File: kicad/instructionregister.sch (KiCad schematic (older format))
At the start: 11 parts, among them U15 74LS173, U16 74LS173, U17 74LS245

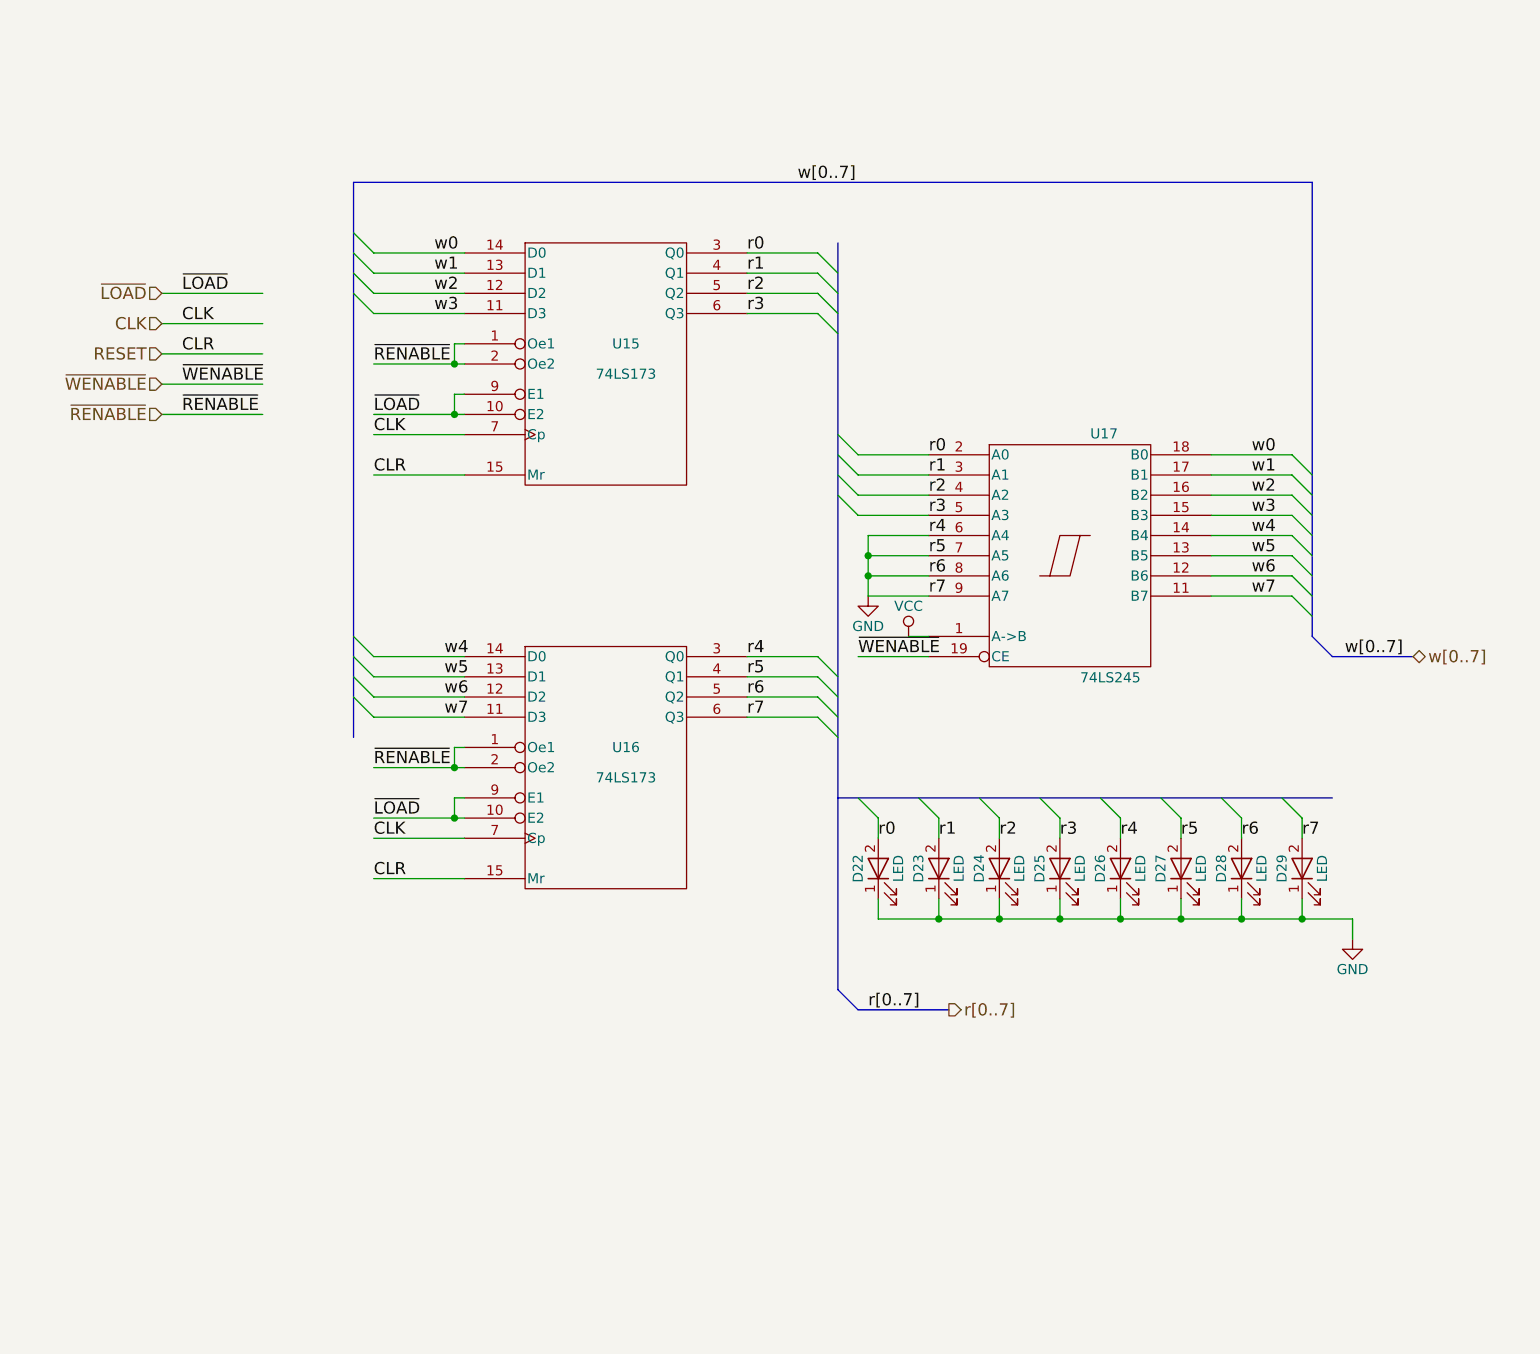
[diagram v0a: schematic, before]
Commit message: Update to current kicad libraries
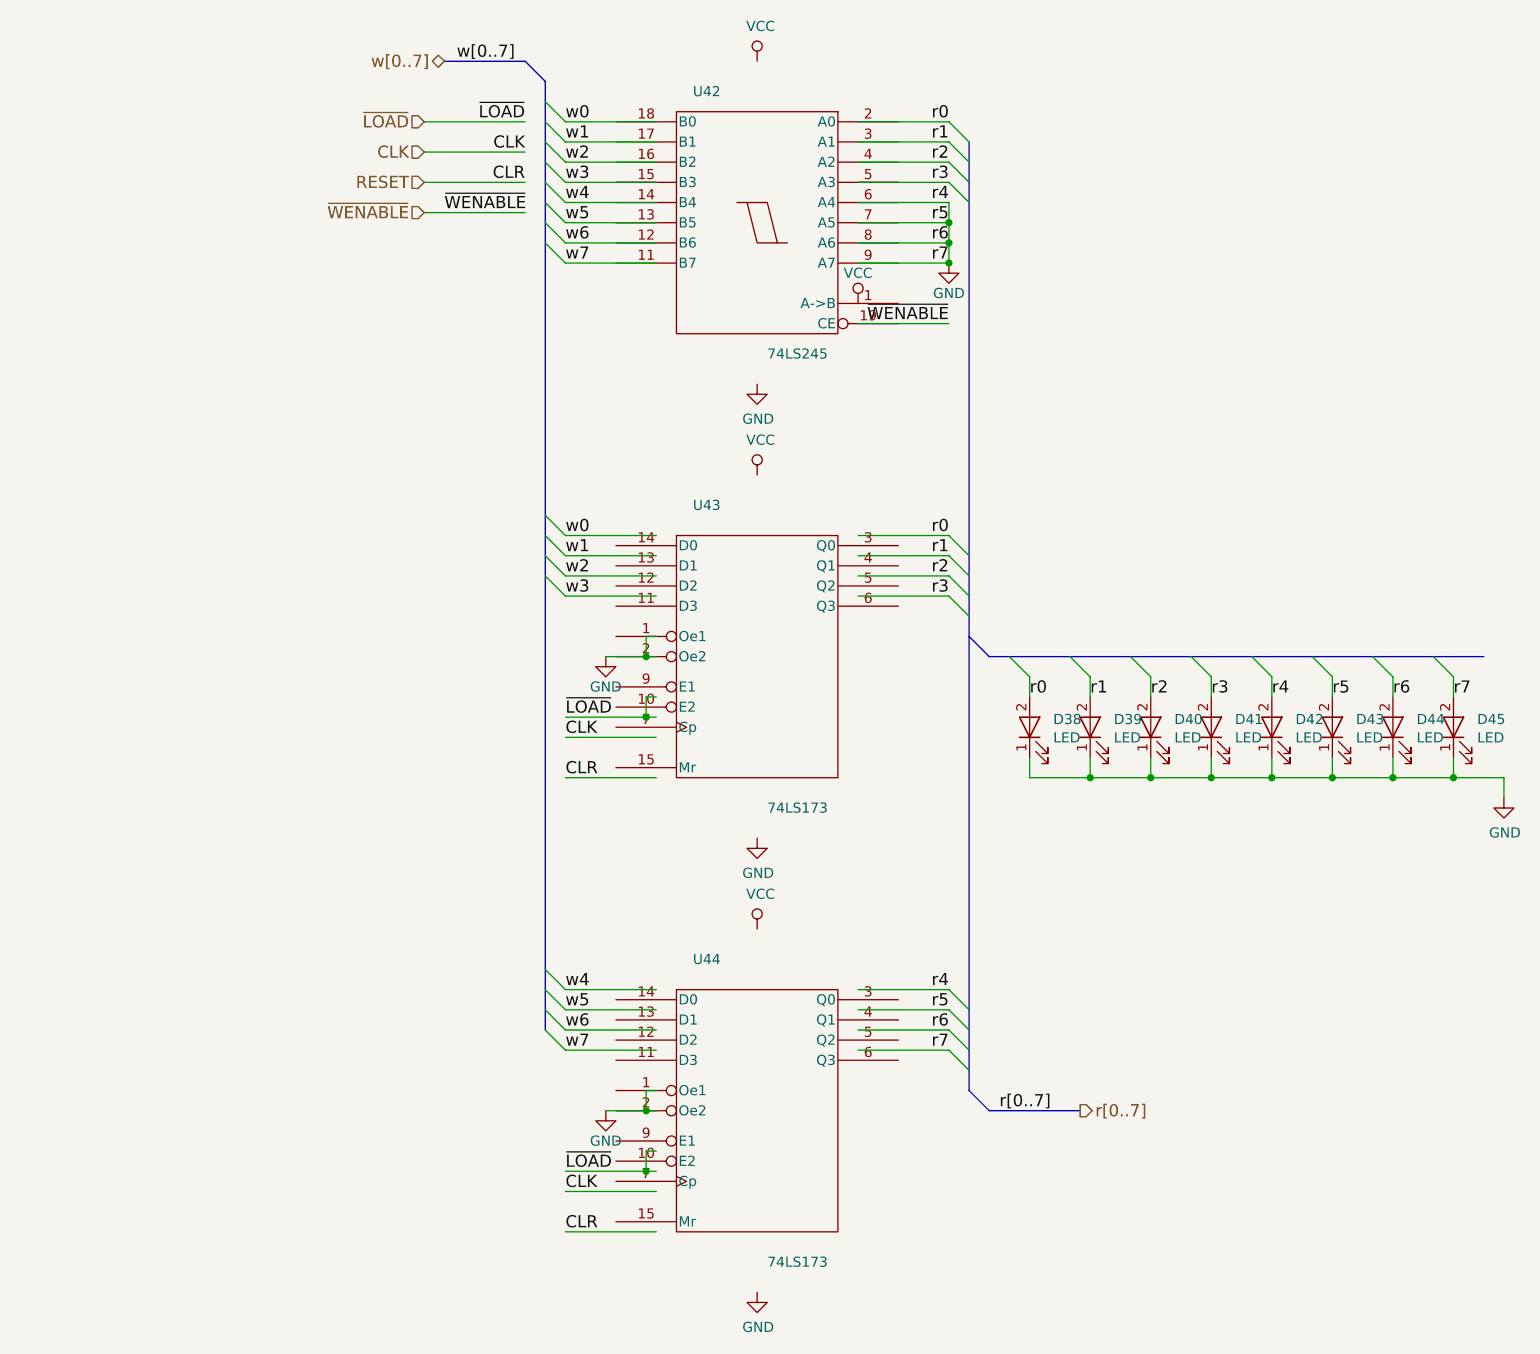
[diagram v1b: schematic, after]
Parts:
- removed D22, D23, D24, D25, D26, D27, D28, D29: LED, LEDs:LED-5MM, symbol LED
- removed U15, U16: 74LS173, Housings_DIP:DIP-16_W7.62mm_LongPads, symbol 74LS173
- removed U17: 74LS245, Housings_DIP:DIP-20_W7.62mm_LongPads, symbol 74LS245
- added D38, D39, D40, D41, D42, D43, D44, D45: LED, symbol Device:LED
- added U42: 74LS245, symbol 74xx:74LS245
- added U43, U44: 74LS173, symbol 74xx:74LS173
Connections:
- net labels removed: ~RENABLE
- wire segments 74 -> 85
